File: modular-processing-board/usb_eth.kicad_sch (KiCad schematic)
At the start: 15 parts, among them J401 TF01A, J801 TYPE-C-31-M-12, U401 SRV05-4

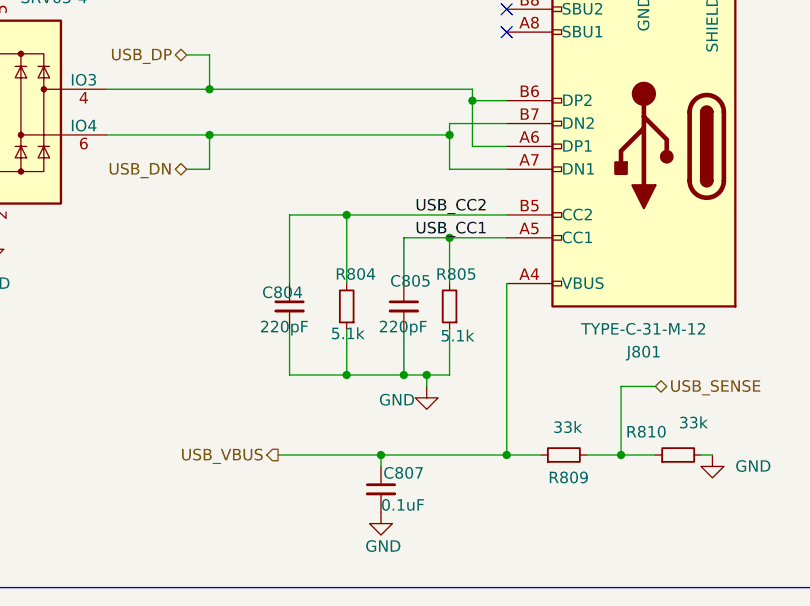
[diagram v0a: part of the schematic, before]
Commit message: completed schematic + layout (next) do footprint checks etc.
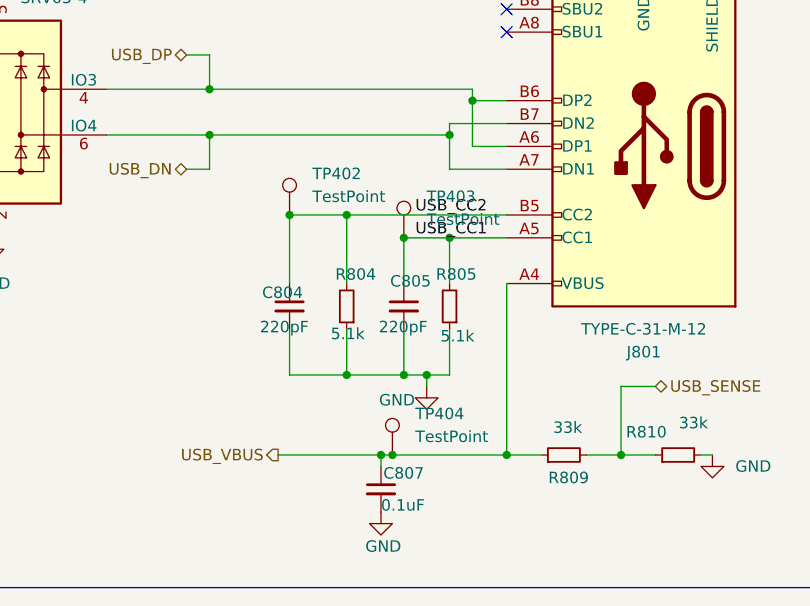
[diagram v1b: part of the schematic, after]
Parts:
- added TP402, TP403, TP404: TestPoint, iw-misc:TestPoint_Pad_D0.5mm, symbol Connector:TestPoint
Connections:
- net USB_CC1: now also TP403.1
- net USB_CC2: now also TP402.1
- net USB_VBUS: now also TP404.1
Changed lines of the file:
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@@
 	)
 	(junction
+		(at 224.79 110.49)
+		(diameter 0)
+		(color 0 0 0 0)
+	)
+	(junction
 		(at 219.71 101.6)
 		(diameter 0)
@@
 	)
 	(junction
+		(at 213.36 83.82)
+		(diameter 0)
+		(color 0 0 0 0)
+	)
+	(junction
 		(at 81.28 80.01)
 		(diameter 0)
@@
 		(color 0 0 0 0)
 	)
+	(junction
+		(at 226.06 86.36)
+		(diameter 0)
+		(color 0 0 0 0)
+	)
 	(no_connect
 		(at 167.64 74.93)
@@
 	(wire
 		(pts
-			(xy 223.52 110.49) (xy 237.49 110.49)
+			(xy 223.52 110.49) (xy 224.79 110.49)
 		)
 		(stroke
@@
 	(wire
 		(pts
+			(xy 224.79 110.49) (xy 237.49 110.49)
+		)
+		(stroke
+			(width 0)
+			(type default)
+		)
+	)
+	(wire
+		(pts
 			(xy 78.74 87.63) (xy 83.82 87.63)
 		)
@@
 	)
 	(symbol
+		(lib_id "Connector:TestPoint")
+		(at 224.79 110.49 0)
+		(unit 1)
+		(exclude_from_sim no)
+		(in_bom yes)
+		(on_board yes)
+		(dnp no)
+		(fields_autoplaced yes)
+		(property "Reference" "TP404"
+			(at 227.33 105.9179 0)
+			(effects
+				(font
+					(size 1.27 1.27)
+				)
+				(justify left)
+			)
+		)
+		(property "Value" "TestPoint"
+			(at 227.33 108.4579 0)
+			(effects
+				(font
+					(size 1.27 1.27)
+				)
+				(justify left)
+			)
+		)
+		(property "Footprint" "iw-misc:TestPoint_Pad_D0.5mm"
+			(at 229.87 110.49 0)
+			(effects
+				(font
+					(size 1.27 1.27)
+				)
+				(hide yes)
+			)
+		)
+		(property "Datasheet" "~"
+			(at 229.87 110.49 0)
+			(effects
+				(font
+					(size 1.27 1.27)
+				)
+				(hide yes)
+			)
+		)
+		(property "Description" "test point"
+			(at 224.79 110.49 0)
+			(effects
+				(font
+					(size 1.27 1.27)
+				)
+				(hide yes)
+			)
+		)
+		(pin "1"
+		)
+		(instances
+			(project "modular-processing-board"
+				(path "/73b5a92f-908b-4f97-a96c-14ee20a7f293/5a39632a-7d64-4b17-8b3b-2384b46c7599"
+					(reference "TP404")
+					(unit 1)
+				)
+			)
+		)
+	)
+	(symbol
 		(lib_id "Device:R_Small")
 		(at 243.84 110.49 90)
@@
 	)
 	(symbol
+		(lib_id "Connector:TestPoint")
+		(at 226.06 86.36 0)
+		(unit 1)
+		(exclude_from_sim no)
+		(in_bom yes)
+		(on_board yes)
+		(dnp no)
+		(fields_autoplaced yes)
+		(property "Reference" "TP403"
+			(at 228.6 81.7879 0)
+			(effects
+				(font
+					(size 1.27 1.27)
+				)
+				(justify left)
+			)
+		)
+		(property "Value" "TestPoint"
+			(at 228.6 84.3279 0)
+			(effects
+				(font
+					(size 1.27 1.27)
+				)
+				(justify left)
+			)
+		)
+		(property "Footprint" "iw-misc:TestPoint_Pad_D0.5mm"
+			(at 231.14 86.36 0)
+			(effects
+				(font
+					(size 1.27 1.27)
+				)
+				(hide yes)
+			)
+		)
+		(property "Datasheet" "~"
+			(at 231.14 86.36 0)
+			(effects
+				(font
+					(size 1.27 1.27)
+				)
+				(hide yes)
+			)
+		)
+		(property "Description" "test point"
+			(at 226.06 86.36 0)
+			(effects
+				(font
+					(size 1.27 1.27)
+				)
+				(hide yes)
+			)
+		)
+		(pin "1"
+		)
+		(instances
+			(project "modular-processing-board"
+				(path "/73b5a92f-908b-4f97-a96c-14ee20a7f293/5a39632a-7d64-4b17-8b3b-2384b46c7599"
+					(reference "TP403")
+					(unit 1)
+				)
+			)
+		)
+	)
+	(symbol
 		(lib_id "Device:C_Small")
 		(at 226.06 93.98 0)
@@
 					(unit 1)
 				)
+			)
+		)
+	)
+	(symbol
+		(lib_id "Connector:TestPoint")
+		(at 213.36 83.82 0)
+		(unit 1)
+		(exclude_from_sim no)
+		(in_bom yes)
+		(on_board yes)
+		(dnp no)
+		(fields_autoplaced yes)
+		(property "Reference" "TP402"
+			(at 215.9 79.2479 0)
+			(effects
+				(font
+					(size 1.27 1.27)
+				)
+				(justify left)
+			)
+		)
+		(property "Value" "TestPoint"
+			(at 215.9 81.7879 0)
+			(effects
+				(font
+					(size 1.27 1.27)
+				)
+				(justify left)
+			)
+		)
+		(property "Footprint" "iw-misc:TestPoint_Pad_D0.5mm"
+			(at 218.44 83.82 0)
+			(effects
+				(font
+					(size 1.27 1.27)
+				)
+				(hide yes)
+			)
+		)
+		(property "Datasheet" "~"
+			(at 218.44 83.82 0)
+			(effects
+				(font
+					(size 1.27 1.27)
+				)
+				(hide yes)
+			)
+		)
+		(property "Description" "test point"
+			(at 213.36 83.82 0)
+			(effects
+				(font
+					(size 1.27 1.27)
+				)
+				(hide yes)
+			)
+		)
+		(pin "1"
+		)
+		(instances
+			(project "modular-processing-board"
+				(path "/73b5a92f-908b-4f97-a96c-14ee20a7f293/5a39632a-7d64-4b17-8b3b-2384b46c7599"
+					(reference "TP402")
+					(unit 1)
+				)
